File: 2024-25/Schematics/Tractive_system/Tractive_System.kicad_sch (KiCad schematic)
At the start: 22 parts, among them J1 Conn_01x03_Pin, J13 Conn_01x03_Pin, J14 BU-P72930-0, J15 UPCR012ALS2, J16 UPCR012ALS1, J17 EM30MSD-A(06), J18 1-66103-8, J19 1-66399-0, J4 UPCR012ALS2, J5 Conn_01x02_Pin, J6 UPCR012ALS1, J7 Conn_01x02_Socket, J8 MSDXLF000F, J9 MSDXLM000

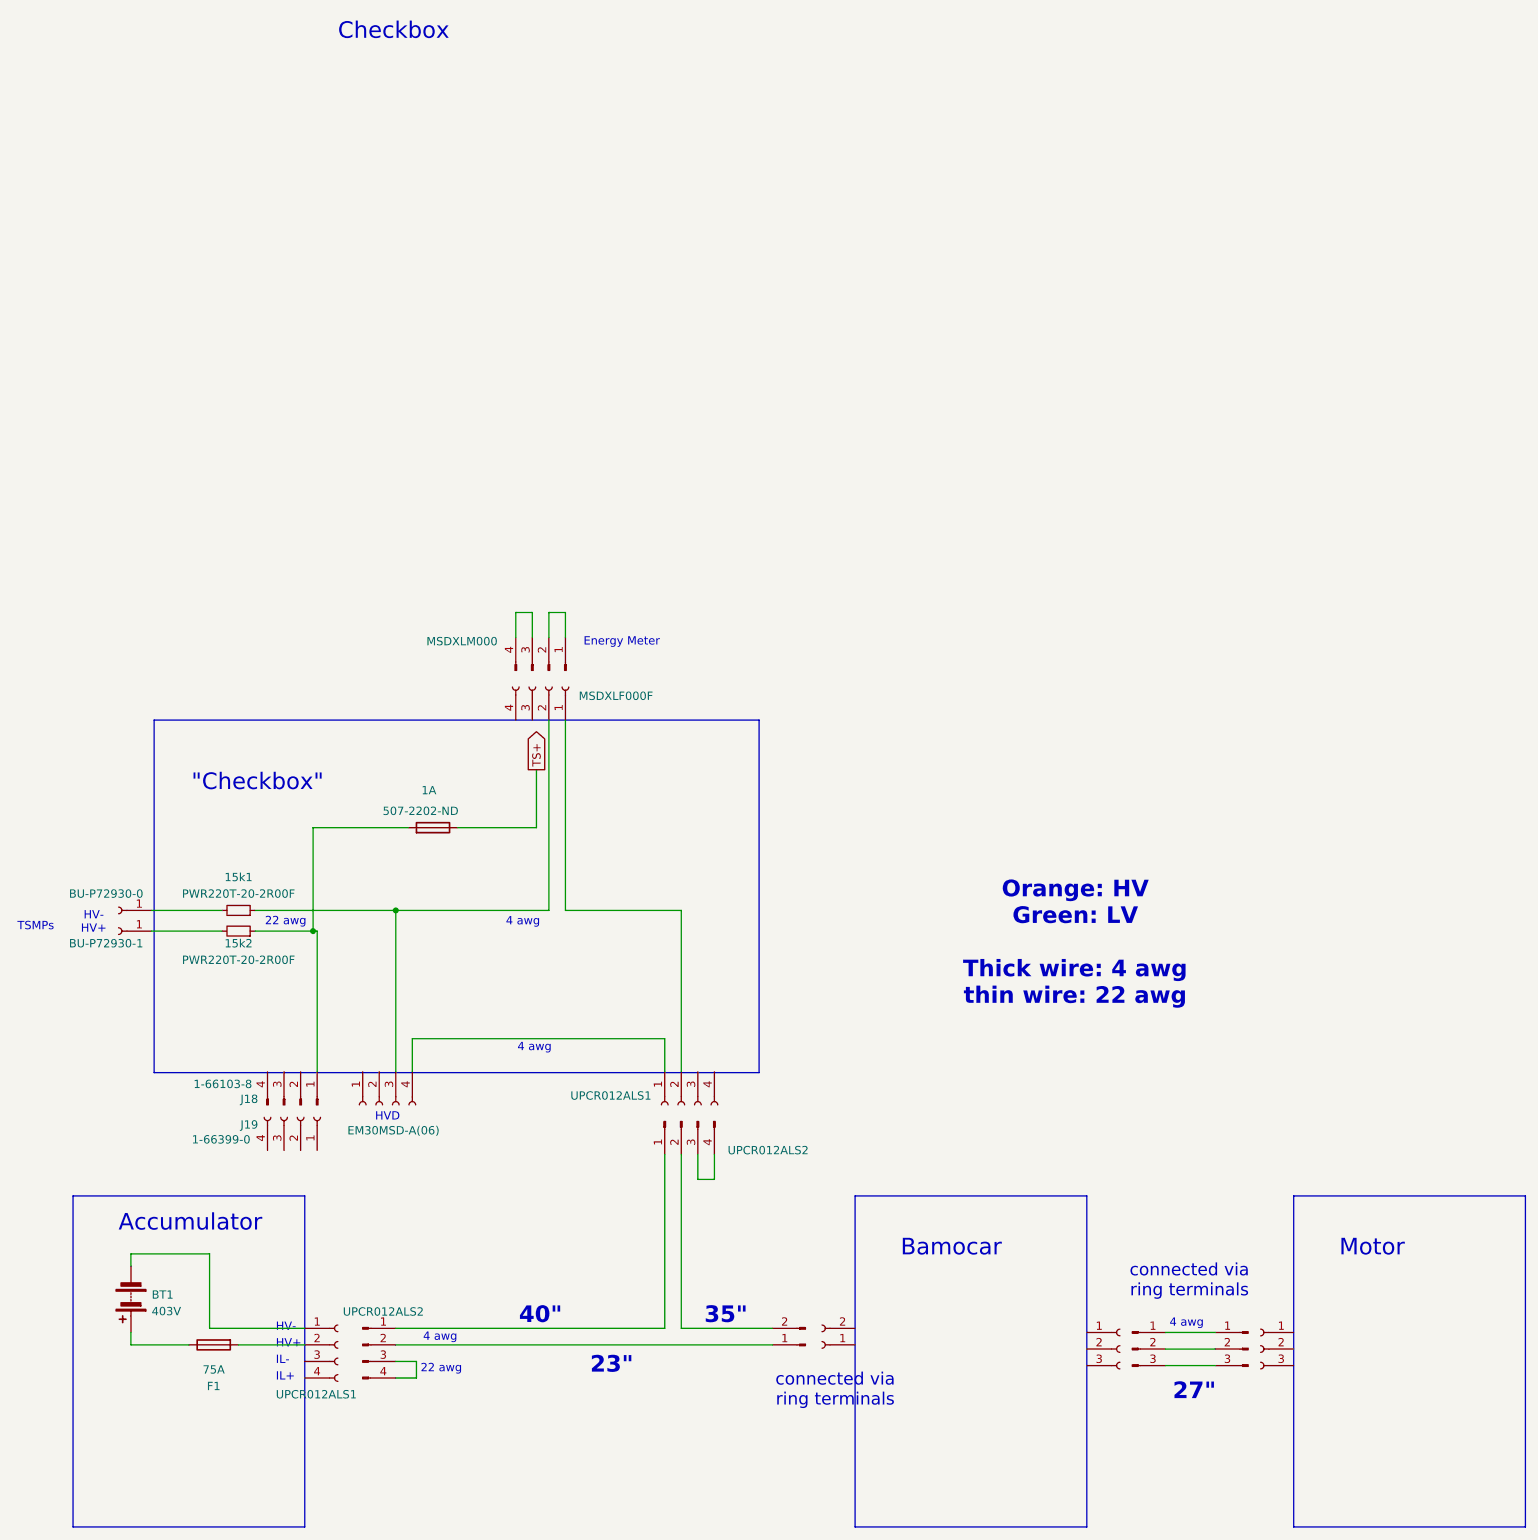
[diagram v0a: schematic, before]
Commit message: integration cleanups
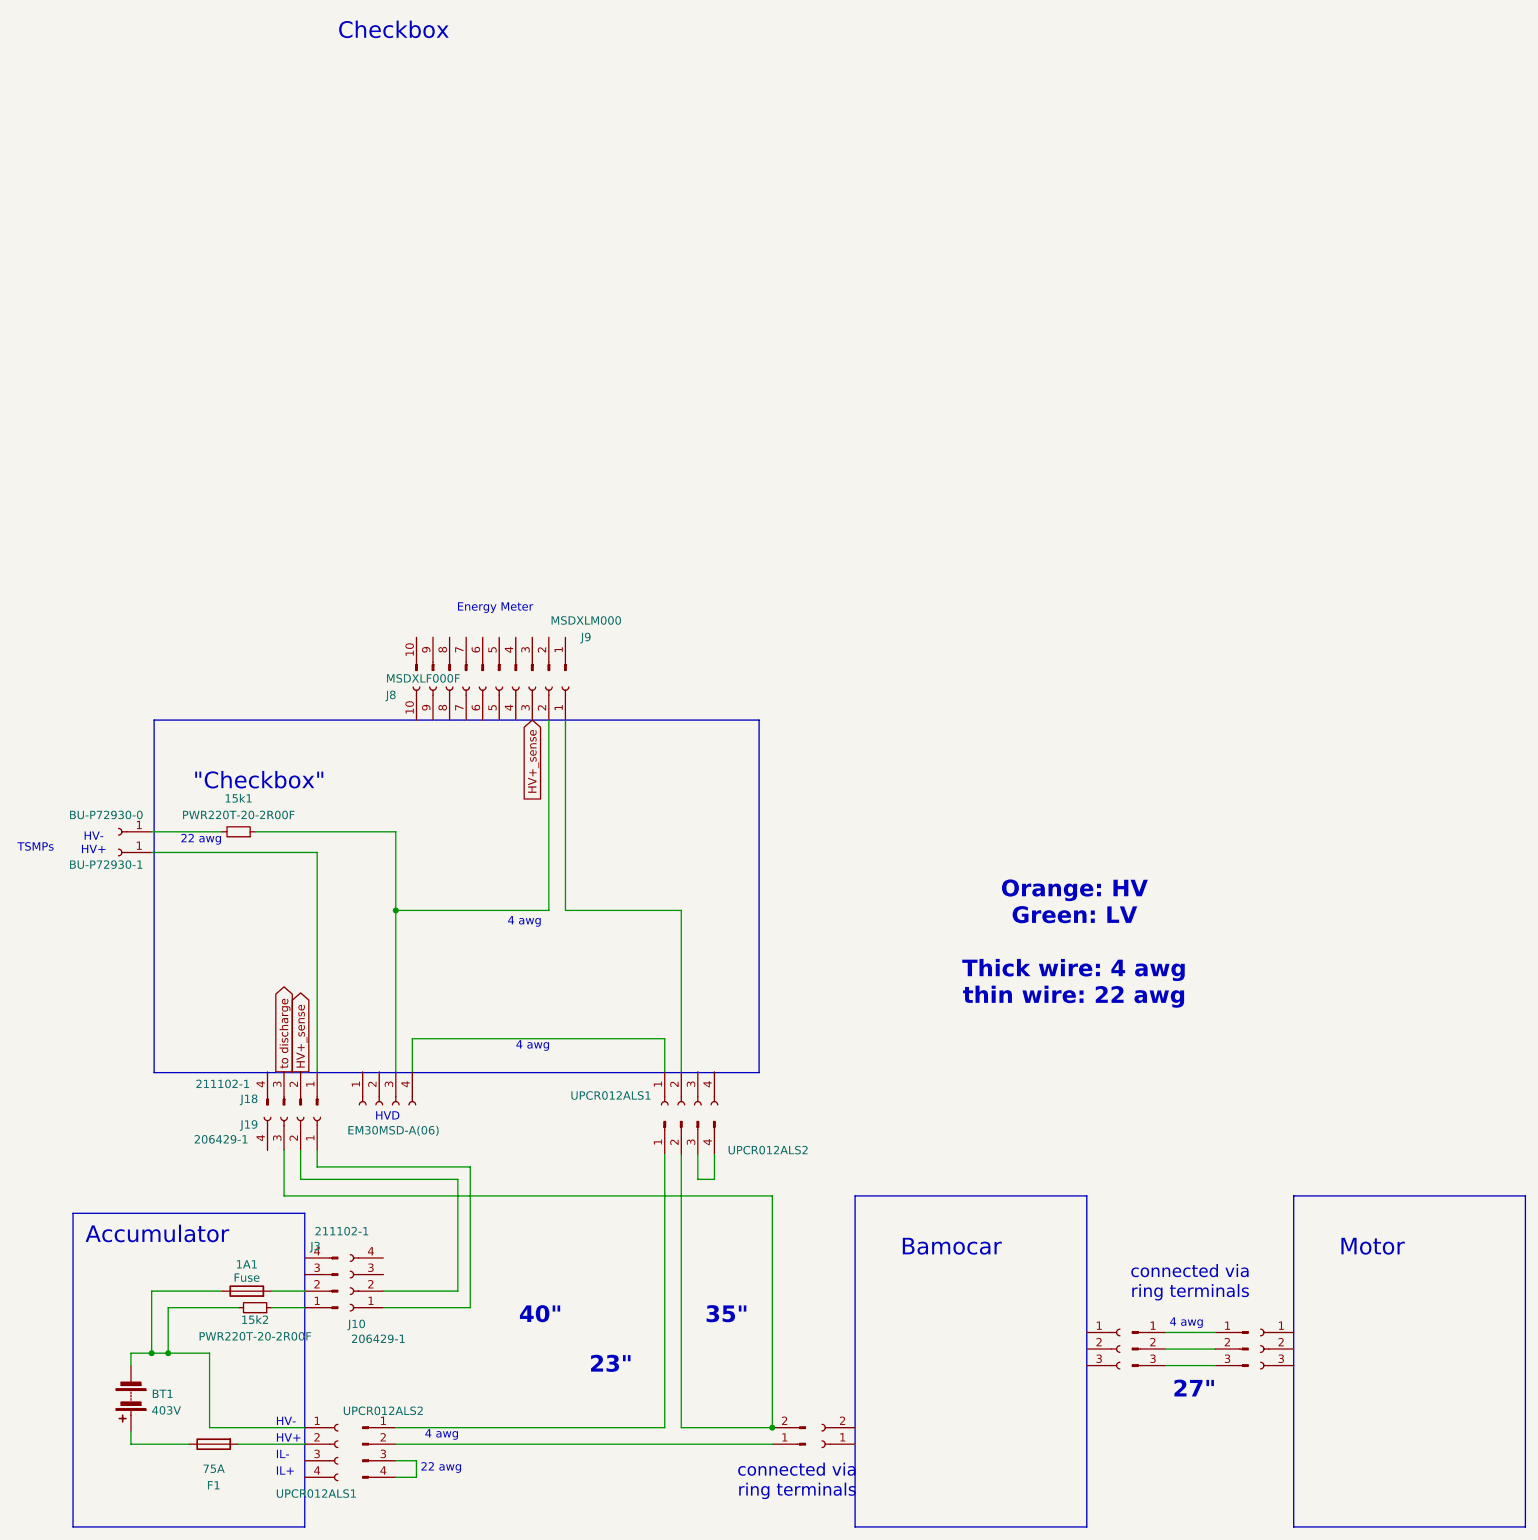
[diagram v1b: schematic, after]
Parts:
- removed 1A: 507-2202-ND, symbol Device:Fuse
- removed J8: MSDXLF000F, symbol Connector:Conn_01x04_Socket
- removed J9: MSDXLM000, symbol Connector:Conn_01x04_Pin
- added 1A1: Fuse, symbol Device:Fuse
- added J10: 206429-1, symbol Connector:Conn_01x04_Socket
- added J3: 211102-1, symbol Connector:Conn_01x04_Pin
- added J8: MSDXLF000F, symbol Connector:Conn_01x10_Socket
- added J9: MSDXLM000, symbol Connector:Conn_01x10_Pin
- J18: value 1-66103-8 -> 211102-1
- J19: value 1-66399-0 -> 206429-1
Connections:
- net at J16.2 (Pin_2): now also J8.1 (Pin_1)
- net at 15k1.1, J17.3 (Pin_3): now also J8.2 (Pin_2)
- net at J15.2 (Pin_2), J5.2 (Pin_2): now also J19.3 (Pin_3)
- net at BT1.2 (-), J6.1 (Pin_1): now also 15k2.2, 1A1.1
- net at 15k2.1: now also J3.1 (Pin_1); no longer J18.1 (Pin_1)
- net at BU-P72930-1.1 (Pin_1): now also J18.1 (Pin_1); no longer 15k2.2
- net at J19.1 (Pin_1): now also J10.1 (Pin_1)
- net at J19.2 (Pin_2): now also J10.2 (Pin_2)
- net HV+_sense: now reaches J18.2 (Pin_2)
- net HV+_sense: now also J8.3 (Pin_3)
- net to discharge: now reaches J18.3 (Pin_3)
- new net: 1A1.2, J3.2 (Pin_2)
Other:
- moved on the sheet: 15k1, BT1, BU-P72930-1, F1
